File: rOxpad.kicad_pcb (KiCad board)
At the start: 2 copper layers, 77.8 x 67.5 mm, 22 parts, among them SW1 SW_Push, U1 ATmega32U4-A, Y1 16MHz

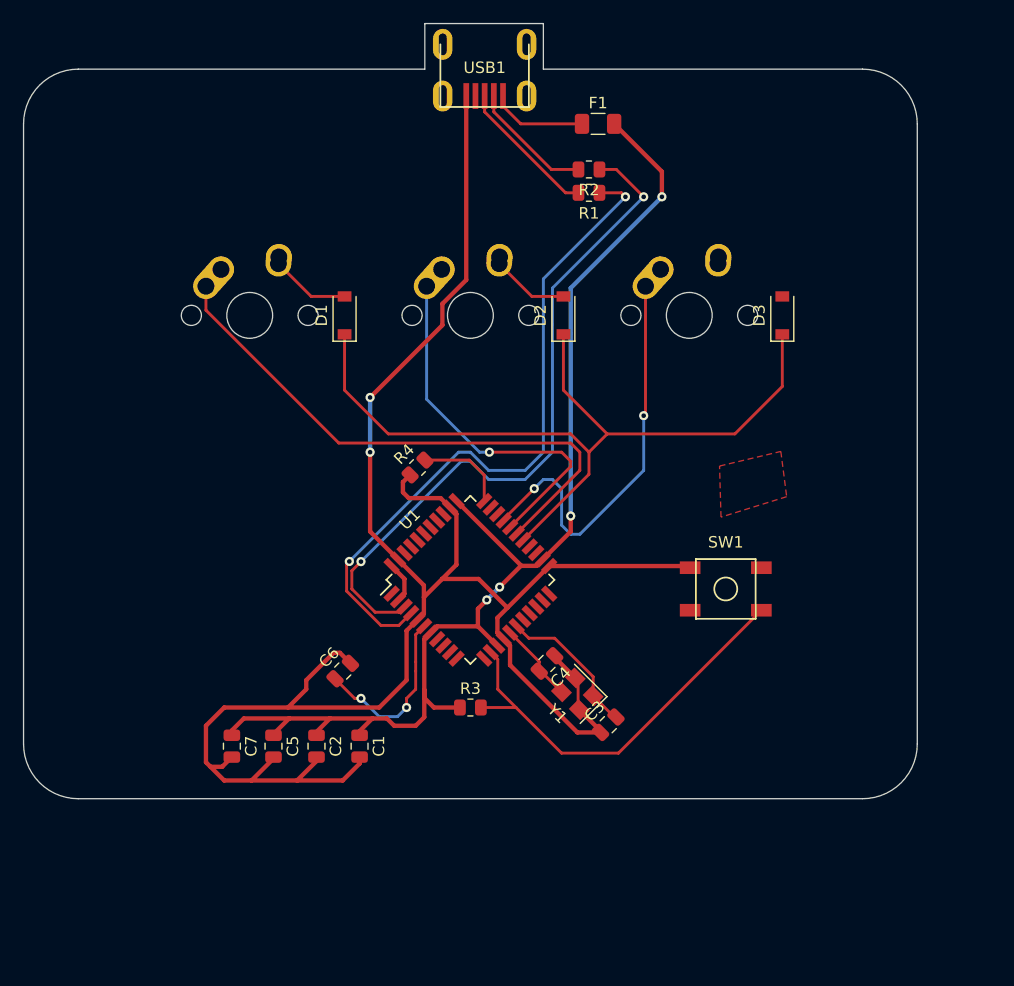
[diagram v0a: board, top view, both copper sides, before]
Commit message: I think it's finished wohoo
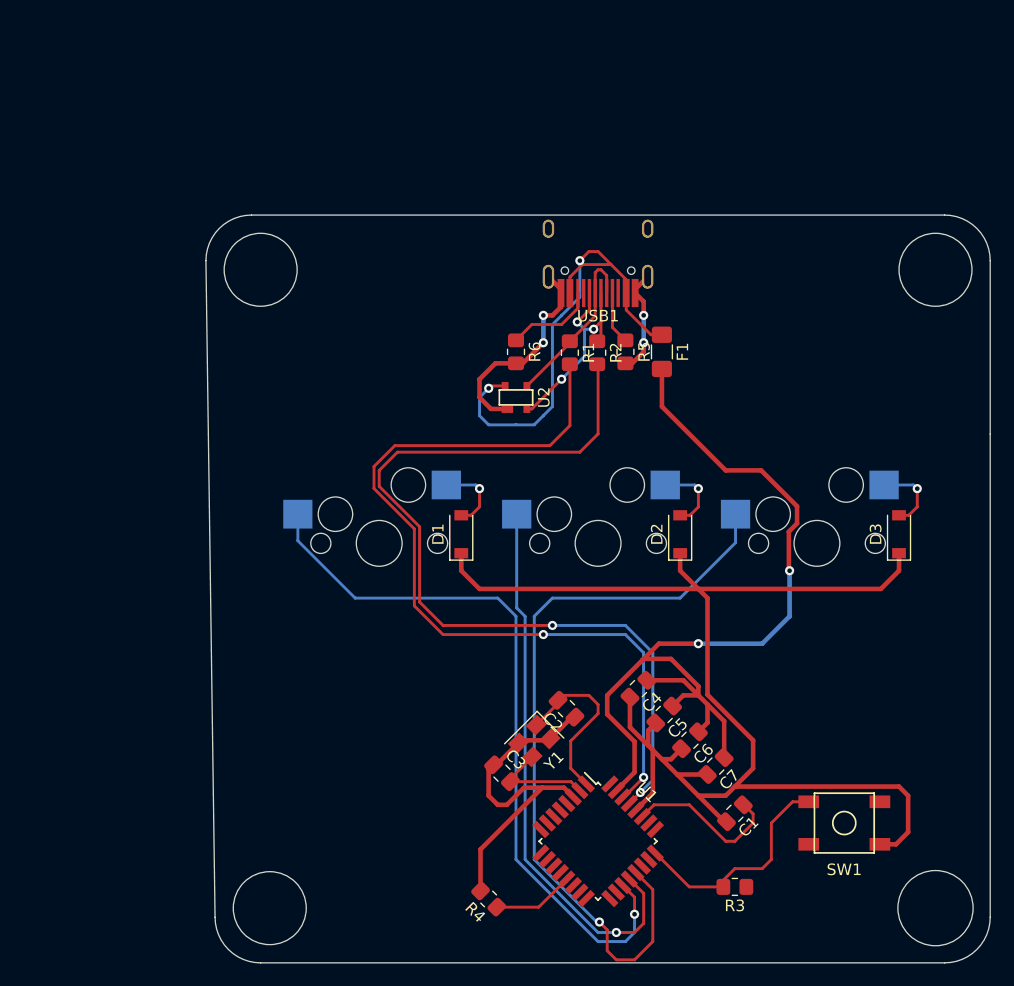
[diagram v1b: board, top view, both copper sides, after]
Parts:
- added R5: 5.1k, Resistor_SMD:R_0805_2012Metric_Pad1.20x1.40mm_HandSolder, F.Cu at (109.5, 72.2)
- added R6: 5.1k, Resistor_SMD:R_0805_2012Metric_Pad1.20x1.40mm_HandSolder, F.Cu at (100.0, 72.2)
- added U2: PRTR5V0U2X, random-keyboard-parts:SOT143B, F.Cu at (100.0, 76.2)
- C1: value 0.1uF -> 1uF; footprint Capacitor_SMD:C_0805_2012Metric -> Capacitor_SMD:C_0805_2012Metric_Pad1.18x1.45mm_HandSolder
- C2: value 0.1uF -> 22Pf; footprint Capacitor_SMD:C_0805_2012Metric -> Capacitor_SMD:C_0805_2012Metric_Pad1.18x1.45mm_HandSolder
- C3, C5: footprint Capacitor_SMD:C_0805_2012Metric -> Capacitor_SMD:C_0805_2012Metric_Pad1.18x1.45mm_HandSolder
- C4: value 22Pf -> 0.1uF; footprint Capacitor_SMD:C_0805_2012Metric -> Capacitor_SMD:C_0805_2012Metric_Pad1.18x1.45mm_HandSolder
- C6: value 1uF -> 0.1uF; footprint Capacitor_SMD:C_0805_2012Metric -> Capacitor_SMD:C_0805_2012Metric_Pad1.18x1.45mm_HandSolder
- C7: value 0.1uF -> 10uF; footprint Capacitor_SMD:C_0805_2012Metric -> Capacitor_SMD:C_0805_2012Metric_Pad1.18x1.45mm_HandSolder
- F1: value 500mA -> Polyfuse_Small; footprint Fuse:Fuse_1206_3216Metric -> Fuse:Fuse_1206_3216Metric_Pad1.42x1.75mm_HandSolder
- MX1, MX2, MX3: footprint MX_Alps_Hybrid:MX-1U-NoLED -> MX_Only:MXOnly-1U-Hotswap
- R1, R2, R3, R4: footprint Resistor_SMD:R_0805_2012Metric -> Resistor_SMD:R_0805_2012Metric_Pad1.20x1.40mm_HandSolder
- U1: value ATmega32U4-A -> ATmega16U2-A; footprint Package_QFP:TQFP-44_10x10mm_P0.8mm -> Package_QFP:TQFP-32_7x7mm_P0.8mm
- USB1: value Molex-0548190589 -> HRO-TYPE-C-31-M-12; footprint random-keyboard-parts:Molex-0548190589 -> Type-C:HRO-TYPE-C-31-M-12-HandSoldering
- moved C7 42.2 mm to (117.4, 108.3), turned to -135 degrees
- moved R4 38.1 mm to (97.6, 119.9), turned to 135 degrees
- moved C5 34.1 mm to (112.9, 103.8), turned to -135 degrees
- moved C1 33.2 mm to (119.1, 112.4), turned to -135 degrees
- moved C6 30.8 mm to (115.2, 106.0), turned to -135 degrees
- moved R3 27.8 mm to (119.1, 118.8), turned to 180 degrees
- moved U1 25.3 mm to (107.2, 114.8), turned to -45 degrees
- moved SW1 22.8 mm to (128.6, 113.2), turned to 0 degrees
- moved MX1 22.8 mm to (88.1, 88.9)
- moved MX2 22.7 mm to (107.2, 88.9)
- moved MX3 22.7 mm to (126.2, 88.9)
- moved C2 22.0 mm to (104.4, 103.3), turned to 135 degrees
- moved D1 21.6 mm to (95.2, 88.1)
- moved D2 21.6 mm to (114.3, 88.1)
- moved D3 21.6 mm to (133.3, 88.1)
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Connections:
- C1 pad 1: +5V -> Net-(C1-Pad1)
- C2 pad 1: +5V -> GND
- C2 pad 2: GND -> XTAL1
- C3 pad 2: XTAL1 -> XTAL2
- C4 pad 1: GND -> +5V
- C4 pad 2: XTAL2 -> GND
- C6 pad 1: Net-(C6-Pad1) -> +5V
- D1 pad 1: ROW-0 -> GND
- D2 pad 1: ROW-0 -> GND
- D3 pad 1: ROW-0 -> GND
- F1 pad 1: Net-(F1-Pad1) -> VCC
- MX1 pad 1: COL-0 -> KEY-0
- MX2 pad 1: COL-1 -> KEY-1
- MX3 pad 1: COL-2 -> KEY-2
- R4 pad 1: GND -> Net-(R4-Pad1)
- R4 pad 2: Net-(R4-Pad2) -> GND
- U1 pad 1: unconnected-(U1-Pad1) -> XTAL1
- U1 pad 13: Net-(R3-Pad2) -> Net-(R4-Pad1)
- U1 pad 14: +5V -> unconnected-(U1-Pad14)
- U1 pad 15: GND -> unconnected-(U1-Pad15)
- U1 pad 16: XTAL2 -> unconnected-(U1-Pad16)
- U1 pad 17: XTAL1 -> unconnected-(U1-Pad17)
- U1 pad 19: unconnected-(U1-Pad19) -> KEY-0
- U1 pad 2: +5V -> XTAL2
- U1 pad 20: unconnected-(U1-Pad20) -> KEY-1
- U1 pad 21: unconnected-(U1-Pad21) -> KEY-2
- U1 pad 23: GND -> unconnected-(U1-Pad23)
- U1 pad 24: +5V -> Net-(R3-Pad2)
- U1 pad 27: ROW-0 -> Net-(C1-Pad1)
- U1 pad 28: COL-0 -> GND
- U1 pad 29: COL-1 -> Net-(R2-Pad2)
- U1 pad 3: Net-(R1-Pad2) -> GND
- U1 pad 30: COL-2 -> Net-(R1-Pad2)
- U1 pad 31: unconnected-(U1-Pad31) -> +5V
- U1 pad 32: unconnected-(U1-Pad32) -> +5V
- U1 pad 4: Net-(R2-Pad2) -> +5V
- U1 pad 5: GND -> unconnected-(U1-Pad5)
- U1 pad 6: Net-(C6-Pad1) -> unconnected-(U1-Pad6)
- U1 pad 7: +5V -> unconnected-(U1-Pad7)
- USB1 pad 2: unconnected-(USB1-Pad2) -> VCC
- USB1 pad 3: D+ -> unconnected-(USB1-Pad3)
- USB1 pad 4: D- -> Net-(R5-Pad1)
- USB1 pad 5: Net-(F1-Pad1) -> D-
- USB1 pad 6: unconnected-(USB1-Pad6) -> D+
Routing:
- net ROW-0: track 72.4 -> 0.00 mm
- net KEY-2: track 0.00 -> 66.1 mm, vias 0 -> 1
- net KEY-0: track 0.00 -> 63.3 mm, vias 0 -> 1
- net COL-0: track 49.1 -> 0.00 mm
- net KEY-1: track 0.00 -> 48.0 mm, vias 0 -> 1
- net VCC: track 0.00 -> 42.7 mm, vias 0 -> 2
- net COL-2: track 36.0 -> 0.00 mm, vias 2 -> 0
- net COL-1: track 32.5 -> 0.00 mm, vias 1 -> 0
- net +5V: track 107.0 -> 80.6 mm, vias 4 -> 2
- net Net-(R3-Pad2): track 37.1 -> 19.8 mm
- net Net-(C6-Pad1): track 15.6 -> 0.00 mm, vias 2 -> 0
- net Net-(R2-Pad2): track 59.9 -> 75.5 mm
- net Net-(C1-Pad1): track 0.00 -> 14.0 mm
- net Net-(R1-Pad2): track 60.6 -> 72.5 mm
- net Net-(F1-Pad1): track 8.39 -> 0.00 mm
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- removed copper zone on F.Cu, net GND
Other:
- board size 77.8 x 67.5 mm -> 68.3 x 65.1 mm
